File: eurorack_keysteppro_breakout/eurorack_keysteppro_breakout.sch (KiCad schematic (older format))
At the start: 25 parts, among them J1 AudioJack2_SwitchT, J10 AudioJack2_SwitchT, J11 AudioJack2_SwitchT, J12 AudioJack2_SwitchT, J13 AudioJack2_SwitchT, J14 AudioJack2_SwitchT, J15 AudioJack2_SwitchT, J16 AudioJack2_SwitchT, J17 AudioJack2_SwitchT, J18 Conn_02x08_Odd_Even, J19 AudioJack2_SwitchT, J2 AudioJack2_SwitchT, J20 AudioJack2_SwitchT, J21 AudioJack2_SwitchT, J22 AudioJack2_SwitchT, J23 Conn_02x08_Odd_Even, J24 AudioJack2_SwitchT, J25 AudioJack2_SwitchT, J3 AudioJack2_SwitchT, J4 AudioJack2_SwitchT, J5 AudioJack2_SwitchT, J6 AudioJack2_SwitchT, J7 AudioJack2_SwitchT, J8 AudioJack2_SwitchT, J9 AudioJack2_SwitchT

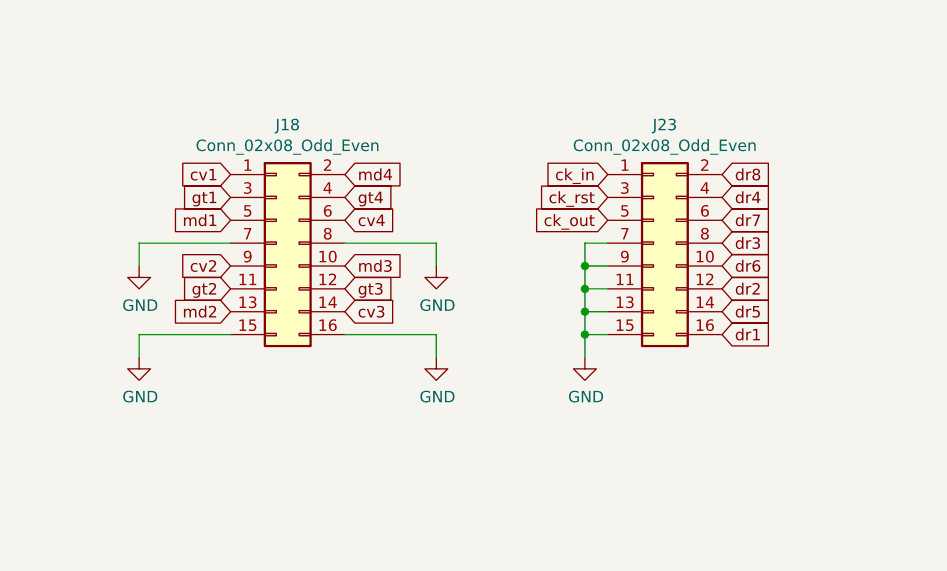
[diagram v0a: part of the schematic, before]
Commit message: some layout
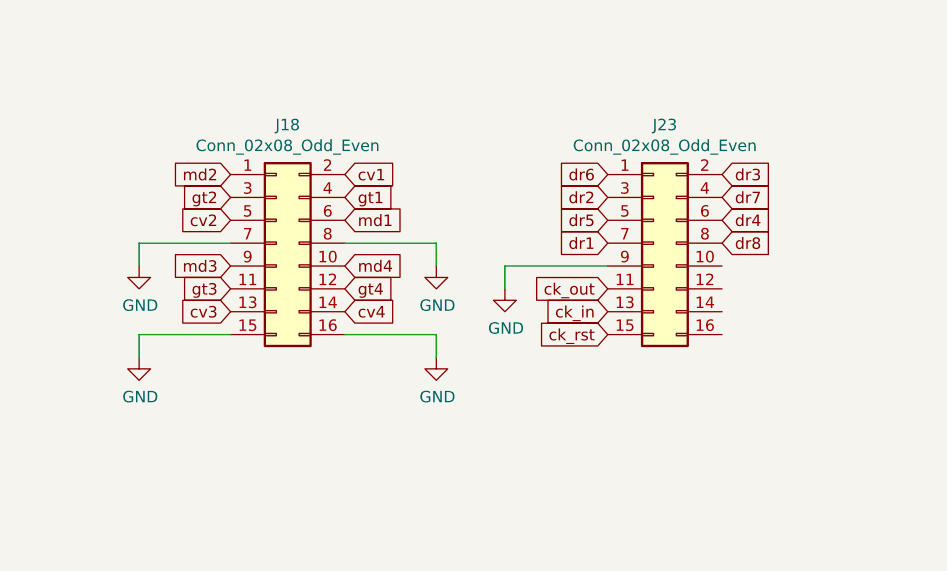
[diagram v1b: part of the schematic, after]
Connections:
- net GND: no longer J23.11 (Pin_11), J23.13 (Pin_13), J23.15 (Pin_15), J23.7 (Pin_7)
- net ck_in: now also J23.13 (Pin_13); no longer J23.1 (Pin_1)
- net ck_out: now also J23.11 (Pin_11); no longer J23.5 (Pin_5)
- net ck_rst: now also J23.15 (Pin_15); no longer J23.3 (Pin_3)
- net cv1: now also J18.2 (Pin_2); no longer J18.1 (Pin_1)
- net cv2: now also J18.5 (Pin_5); no longer J18.9 (Pin_9)
- net cv3: now also J18.13 (Pin_13); no longer J18.14 (Pin_14)
- net cv4: now also J18.14 (Pin_14); no longer J18.6 (Pin_6)
- net dr1: now also J23.7 (Pin_7); no longer J23.16 (Pin_16)
- net dr2: now also J23.3 (Pin_3); no longer J23.12 (Pin_12)
- net dr3: now also J23.2 (Pin_2); no longer J23.8 (Pin_8)
- net dr4: now also J23.6 (Pin_6); no longer J23.4 (Pin_4)
- net dr5: now also J23.5 (Pin_5); no longer J23.14 (Pin_14)
- net dr6: now also J23.1 (Pin_1); no longer J23.10 (Pin_10)
- net dr7: now also J23.4 (Pin_4); no longer J23.6 (Pin_6)
- net dr8: now also J23.8 (Pin_8); no longer J23.2 (Pin_2)
- net gt1: now also J18.4 (Pin_4); no longer J18.3 (Pin_3)
- net gt2: now also J18.3 (Pin_3); no longer J18.11 (Pin_11)
- net gt3: now also J18.11 (Pin_11); no longer J18.12 (Pin_12)
- net gt4: now also J18.12 (Pin_12); no longer J18.4 (Pin_4)
- net md1: now also J18.6 (Pin_6); no longer J18.5 (Pin_5)
- net md2: now also J18.1 (Pin_1); no longer J18.13 (Pin_13)
- net md3: now also J18.9 (Pin_9); no longer J18.10 (Pin_10)
- net md4: now also J18.10 (Pin_10); no longer J18.2 (Pin_2)
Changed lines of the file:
@@
 Wire Wire Line
 	4450 6050 4700 6050
-Text GLabel 7150 4300 0    50   Input ~ 0
+Text GLabel 7650 4300 2    50   Input ~ 0
 cv1
-Text GLabel 7150 4400 0    50   Input ~ 0
+Text GLabel 7650 4400 2    50   Input ~ 0
 gt1
-Text GLabel 7150 4500 0    50   Input ~ 0
+Text GLabel 7650 4500 2    50   Input ~ 0
 md1
 $Comp
@@
 	1    0    0    -1
 $EndComp
+Text GLabel 7150 4500 0    50   Input ~ 0
+cv2
+Text GLabel 7150 4400 0    50   Input ~ 0
+gt2
+Text GLabel 7150 4300 0    50   Input ~ 0
+md2
+Text GLabel 7150 4900 0    50   Input ~ 0
+cv3
+Text GLabel 7150 4800 0    50   Input ~ 0
+gt3
 Text GLabel 7150 4700 0    50   Input ~ 0
-cv2
-Text GLabel 7150 4800 0    50   Input ~ 0
-gt2
-Text GLabel 7150 4900 0    50   Input ~ 0
-md2
+md3
 Text GLabel 7650 4900 2    50   Input ~ 0
-cv3
+cv4
 Text GLabel 7650 4800 2    50   Input ~ 0
-gt3
+gt4
 Text GLabel 7650 4700 2    50   Input ~ 0
-md3
-Text GLabel 7650 4500 2    50   Input ~ 0
-cv4
-Text GLabel 7650 4400 2    50   Input ~ 0
-gt4
-Text GLabel 7650 4300 2    50   Input ~ 0
 md4
+Text GLabel 8800 4900 0    50   Input ~ 0
+ck_in
+Text GLabel 8800 4800 0    50   Input ~ 0
+ck_out
+Text GLabel 8800 5000 0    50   Input ~ 0
+ck_rst
+Text GLabel 8800 4600 0    50   Input ~ 0
+dr1
+Text GLabel 8800 4400 0    50   Input ~ 0
+dr2
+Text GLabel 9300 4300 2    50   Input ~ 0
+dr3
+Text GLabel 9300 4500 2    50   Input ~ 0
+dr4
+Text GLabel 8800 4500 0    50   Input ~ 0
+dr5
 Text GLabel 8800 4300 0    50   Input ~ 0
-ck_in
-Text GLabel 8800 4500 0    50   Input ~ 0
-ck_out
-Text GLabel 8800 4400 0    50   Input ~ 0
-ck_rst
-Text GLabel 9300 5000 2    50   Input ~ 0
-dr1
-Text GLabel 9300 4800 2    50   Input ~ 0
-dr2
+dr6
+Text GLabel 9300 4400 2    50   Input ~ 0
+dr7
 Text GLabel 9300 4600 2    50   Input ~ 0
-dr3
-Text GLabel 9300 4400 2    50   Input ~ 0
-dr4
-Text GLabel 9300 4900 2    50   Input ~ 0
-dr5
-Text GLabel 9300 4700 2    50   Input ~ 0
-dr6
-Text GLabel 9300 4500 2    50   Input ~ 0
-dr7
-Text GLabel 9300 4300 2    50   Input ~ 0
 dr8
 $Comp
@@
 	8050 5000 8050 5100
 $Comp
-L power:GND #PWR024
-U 1 1 61A7AB11
-P 8700 5100
-F 0 "#PWR024" H 8700 4850 50  0001 C CNN
-F 1 "GND" H 8705 4927 50  0000 C CNN
-F 2 "" H 8700 5100 50  0001 C CNN
-F 3 "" H 8700 5100 50  0001 C CNN
-	1    8700 5100
-	1    0    0    -1
-$EndComp
-$Comp
 L Connector:AudioJack2_SwitchT J2
 U 1 1 61AAFD60
@@
 	1    0    0    -1
 $EndComp
-Wire Wire Line
-	8800 4600 8700 4600
-Wire Wire Line
-	8700 4600 8700 4700
-Wire Wire Line
-	8800 4700 8700 4700
-Connection ~ 8700 4700
-Wire Wire Line
-	8700 4700 8700 4800
-Wire Wire Line
-	8800 4800 8700 4800
-Connection ~ 8700 4800
-Wire Wire Line
-	8700 4800 8700 4900
-Wire Wire Line
-	8800 4900 8700 4900
-Connection ~ 8700 4900
-Wire Wire Line
-	8700 4900 8700 5000
-Wire Wire Line
-	8800 5000 8700 5000
-Connection ~ 8700 5000
-Wire Wire Line
-	8700 5000 8700 5100
+$Comp
+L power:GND #PWR0101
+U 1 1 61BBA297
+P 8350 4800
+F 0 "#PWR0101" H 8350 4550 50  0001 C CNN
+F 1 "GND" H 8355 4627 50  0000 C CNN
+F 2 "" H 8350 4800 50  0001 C CNN
+F 3 "" H 8350 4800 50  0001 C CNN
+	1    8350 4800
+	1    0    0    -1
+$EndComp
+Wire Wire Line
+	8350 4800 8350 4700
+Wire Wire Line
+	8800 4700 8350 4700
 $EndSCHEMATC
